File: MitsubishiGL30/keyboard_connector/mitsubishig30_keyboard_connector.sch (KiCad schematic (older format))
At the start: 2 parts, among them J1 CONN_02x13, J2 CONN_02x13

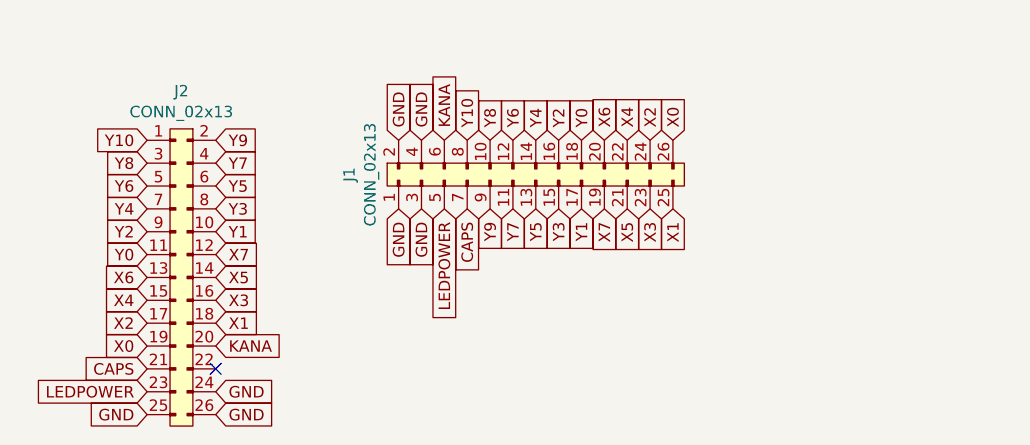
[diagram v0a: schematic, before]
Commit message: Add files via upload
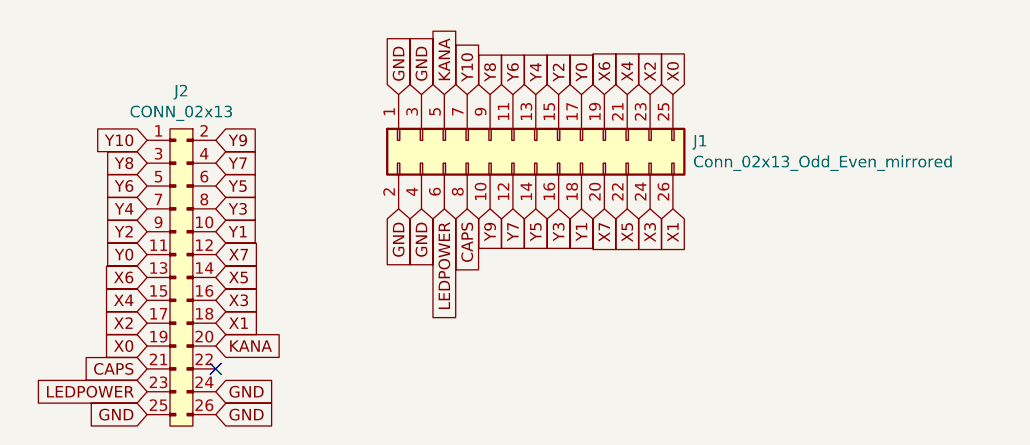
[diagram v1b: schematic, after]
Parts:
- removed J1: CONN_02x13, Connector:26hirosi, symbol agg-kicad:CONN_02x13
- added J1: Conn_02x13_Odd_Even_mirrored, Connector:26hirosi, symbol Connector_Generic:Conn_02x13_Odd_Even_mirrored
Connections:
- net CAPS: now also J1.8 (Pin_8)
- net GND: now also J1.1 (Pin_1), J1.2 (Pin_2), J1.3 (Pin_3), J1.4 (Pin_4)
- net KANA: now also J1.5 (Pin_5)
- net LEDPOWER: now also J1.6 (Pin_6)
- net X0: now also J1.25 (Pin_25)
- net X1: now also J1.26 (Pin_26)
- net X2: now also J1.23 (Pin_23)
- net X3: now also J1.24 (Pin_24)
- net X4: now also J1.21 (Pin_21)
- net X5: now also J1.22 (Pin_22)
- net X6: now also J1.19 (Pin_19)
- net X7: now also J1.20 (Pin_20)
- net Y0: now also J1.17 (Pin_17)
- net Y1: now also J1.18 (Pin_18)
- net Y10: now also J1.7 (Pin_7)
- net Y2: now also J1.15 (Pin_15)
- net Y3: now also J1.16 (Pin_16)
- net Y4: now also J1.13 (Pin_13)
- net Y5: now also J1.14 (Pin_14)
- net Y6: now also J1.11 (Pin_11)
- net Y7: now also J1.12 (Pin_12)
- net Y8: now also J1.9 (Pin_9)
- net Y9: now also J1.10 (Pin_10)
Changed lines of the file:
@@
 	1    0    0    -1
 $EndComp
-$Comp
-L agg-kicad:CONN_02x13 J1
-U 1 1 62095F01
-P 4400 2200
-F 0 "J1" H 4350 2415 50  0000 C CNN
-F 1 "CONN_02x13" H 4350 2324 50  0000 C CNN
-F 2 "Connector:26hirosi" H 4400 2200 50  0001 C CNN
-F 3 "" H 4400 2200 50  0001 C CNN
-	1    4400 2200
-	0    -1   -1   0
-$EndComp
-Text GLabel 5600 2100 1    50   Input ~ 0
+Text GLabel 5600 1900 1    50   Input ~ 0
 X0
-Text GLabel 5500 2100 1    50   Input ~ 0
+Text GLabel 5500 1900 1    50   Input ~ 0
 X2
-Text GLabel 5400 2100 1    50   Input ~ 0
+Text GLabel 5400 1900 1    50   Input ~ 0
 X4
-Text GLabel 5300 2100 1    50   Input ~ 0
+Text GLabel 5300 1900 1    50   Input ~ 0
 X6
-Text GLabel 5200 2100 1    50   Input ~ 0
+Text GLabel 5200 1900 1    50   Input ~ 0
 Y0
-Text GLabel 5100 2100 1    50   Input ~ 0
+Text GLabel 5100 1900 1    50   Input ~ 0
 Y2
-Text GLabel 5000 2100 1    50   Input ~ 0
+Text GLabel 5000 1900 1    50   Input ~ 0
 Y4
-Text GLabel 4900 2100 1    50   Input ~ 0
+Text GLabel 4900 1900 1    50   Input ~ 0
 Y6
-Text GLabel 4800 2100 1    50   Input ~ 0
+Text GLabel 4800 1900 1    50   Input ~ 0
 Y8
-Text GLabel 4700 2100 1    50   Input ~ 0
+Text GLabel 4700 1900 1    50   Input ~ 0
 Y10
-Text GLabel 4600 2100 1    50   Input ~ 0
+Text GLabel 4600 1900 1    50   Input ~ 0
 KANA
-Text GLabel 4500 2100 1    50   Input ~ 0
+Text GLabel 4500 1900 1    50   Input ~ 0
 GND
-Text GLabel 4400 2100 1    50   Input ~ 0
+Text GLabel 4400 1900 1    50   Input ~ 0
 GND
 Text GLabel 5600 2400 3    50   Input ~ 0
@@
 GND
 NoConn ~ 3600 3100
+$Comp
+L Connector_Generic:Conn_02x13_Odd_Even_mirrored J1
+U 1 1 6223D473
+P 5050 2150
+F 0 "J1" V 5096 1512 50  0000 R CNN
+F 1 "Conn_02x13_Odd_Even_mirrored" V 5005 1512 50  0000 R CNN
+F 2 "Connector:26hirosi" H 5100 2200 50  0001 C CNN
+F 3 "~" H 5100 2200 50  0001 C CNN
+	1    5050 2150
+	0    -1   -1   0
+$EndComp
 $EndSCHEMATC
